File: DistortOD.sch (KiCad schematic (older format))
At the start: 27 parts

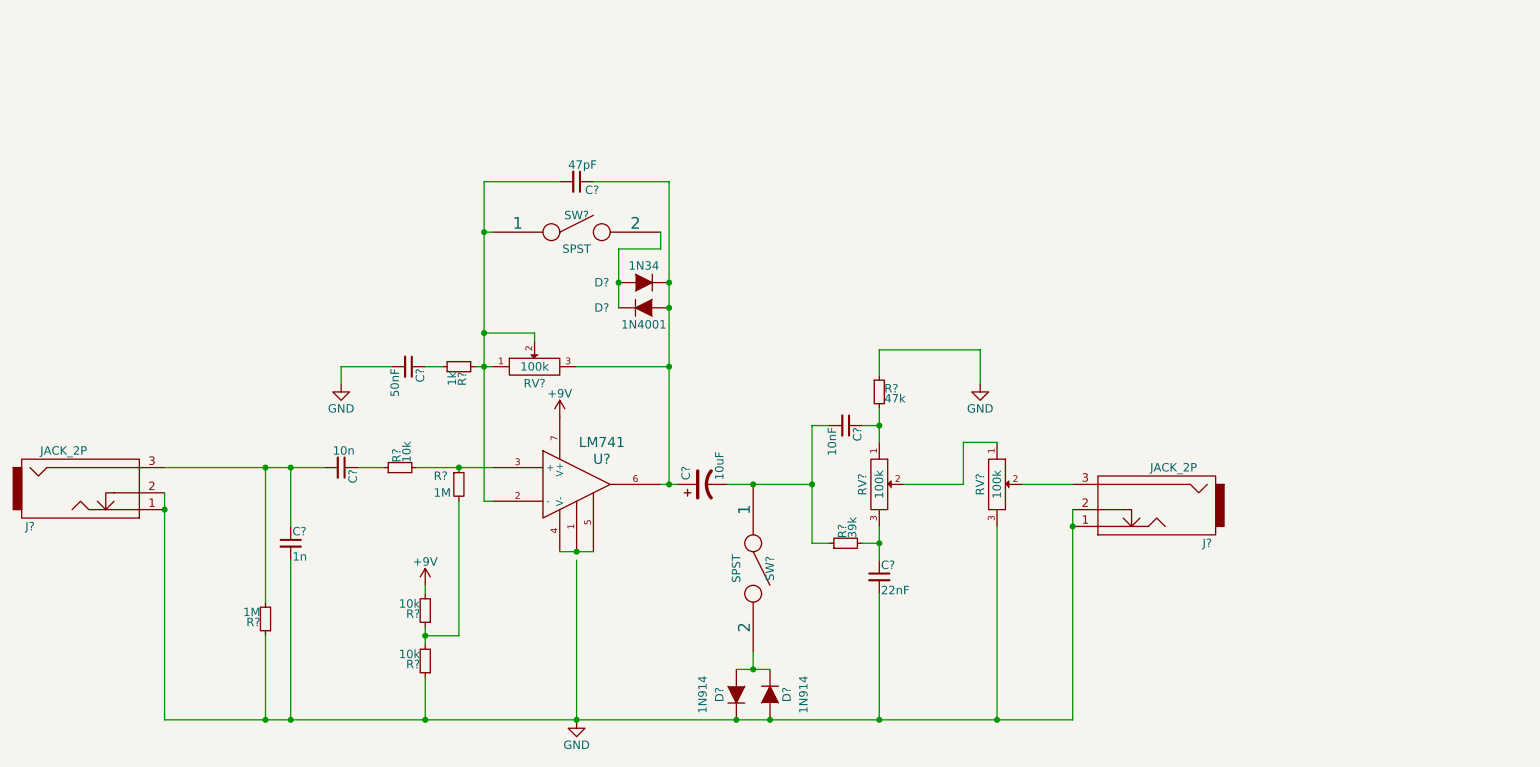
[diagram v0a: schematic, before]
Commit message: add comments and clean up
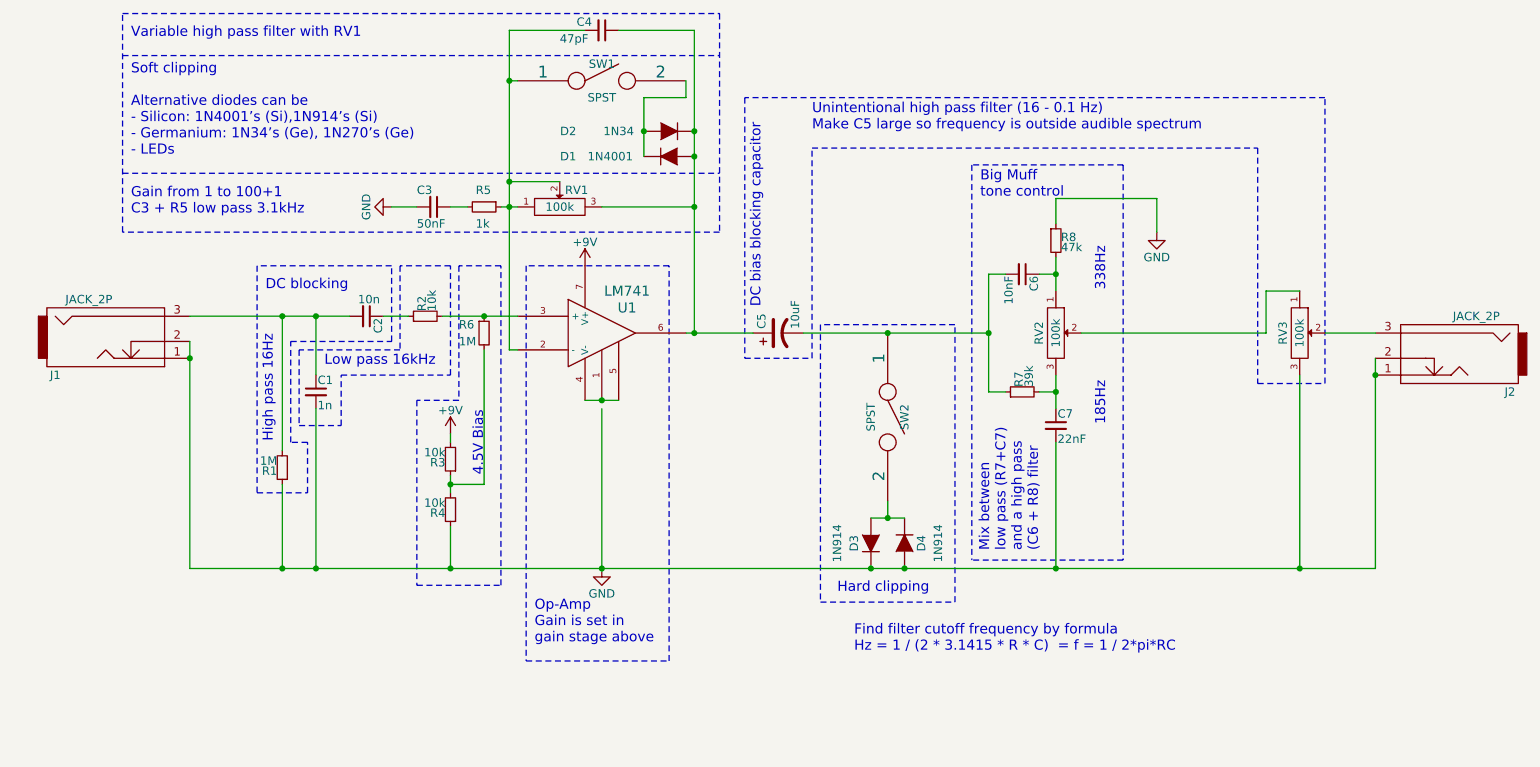
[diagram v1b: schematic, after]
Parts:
- gave numbers to parts that had none: 27
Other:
- note added: "185Hz"
- note added: "338Hz"
- note added: "4.5V Bias"
- note added: "Big Muff \ntone control"
- note added: "DC bias blocking capacitor"
- note added: "DC blocking"
- note added: "Find filter cutoff frequency by formula\nHz = 1 / (2 * 3.1415 * R * C) = f = 1 / 2*pi*RC"
- note added: "Gain from 1 to 100+1\nC3 + R5 low pass 3.1kHz"
- note added: "Hard clipping"
- note added: "High pass 16Hz"
- note added: "Low pass 16kHz"
- note added: "Mix between \nlow pass (R7+C7) \nand a high pass \n(C6 + R8) filter"
- note added: "Op-Amp\nGain is set in \ngain stage above"
- note added: "Soft clipping\n\nAlternative diodes can be\n- Silicon: 1N4001’s (Si),1N914’s (Si)\n- Germanium: 1N34’s (Ge), 1N270’s (Ge)\n- LEDs"
- note added: "Unintentional high pass filter (16 - 0.1 Hz)\nMake C5 large so frequency is outside audible spectrum"
- note added: "Variable high pass filter with RV1"
- moved on the sheet: C1, C2, C3, C4, C5, C6, C7, D1, D2, D3, D4, J1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
